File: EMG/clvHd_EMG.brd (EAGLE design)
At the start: 21 x 18.5 mm, 25 parts, among them J1 XF2J-1824-12, J2 XF2J-1824-12, U1 ADS1293CISQ/NOPB

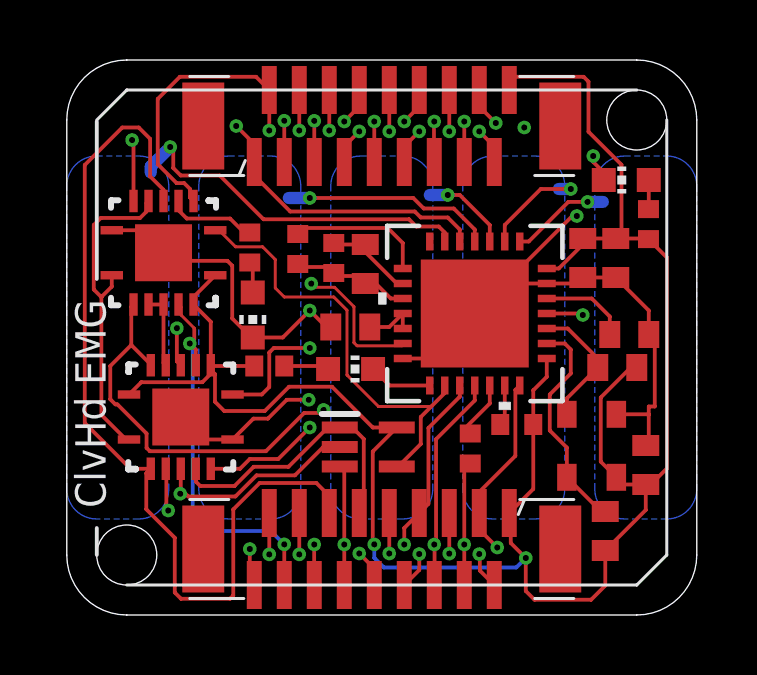
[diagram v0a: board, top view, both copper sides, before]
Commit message: master update
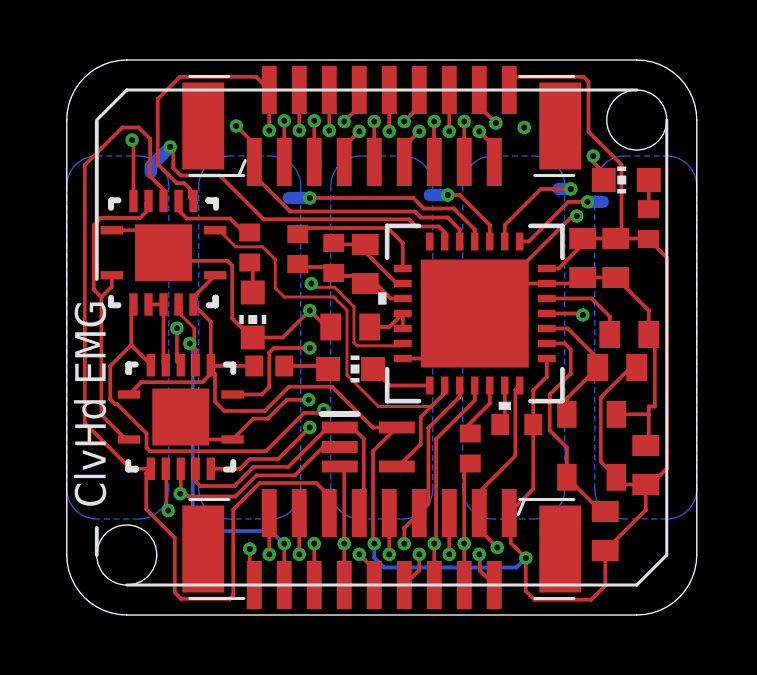
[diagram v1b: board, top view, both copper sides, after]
